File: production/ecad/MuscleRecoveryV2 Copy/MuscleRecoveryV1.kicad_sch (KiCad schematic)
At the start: 18 parts, among them J6 Screw_Terminal_01x06, U6 ESP32-WROOM-32E__16MB_

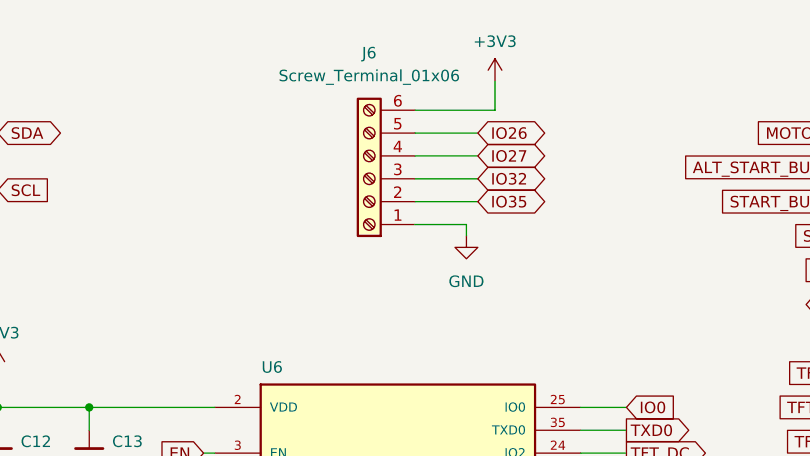
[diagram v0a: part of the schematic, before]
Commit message: Created New Layout
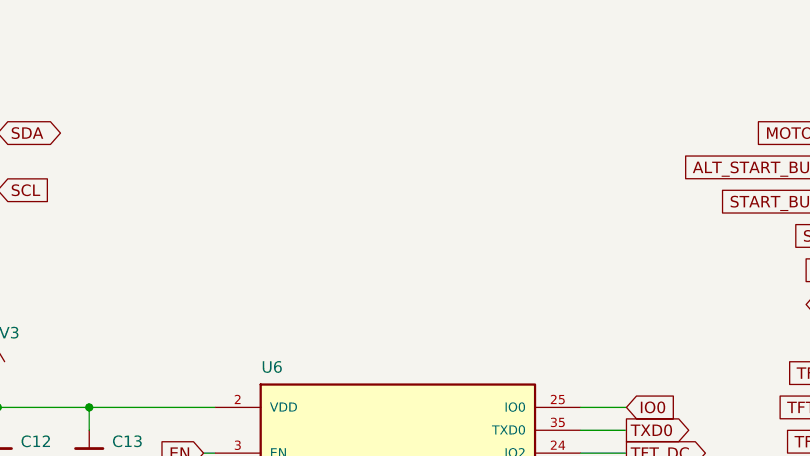
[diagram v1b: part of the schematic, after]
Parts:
- removed J6: Screw_Terminal_01x06, symbol Connector:Screw_Terminal_01x06
- C12, C13: footprint Capacitor_SMD:C_0805_2012Metric -> Capacitor_SMD:C_0402_1005Metric
- R30, R31, R34: footprint Resistor_SMD:R_0805_2012Metric -> Resistor_SMD:R_0402_1005Metric
- U6: footprint ESP32-WROOM-32E__16MB_:XCVR_ESP32-WROOM-32E__16MB_ -> Muscle_Recovery_Footprint_Library:XCVR_ESP32-WROOM-32E__16MB_
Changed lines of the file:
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@@
-    (stroke (width 0) (type default))
-  )
-  (wire (pts (xy 141.605 38.1) (xy 148.59 38.1))
     (stroke (width 0) (type default))
   )
@@
     (stroke (width 0) (type default))
   )
-  (wire (pts (xy 141.605 30.48) (xy 148.59 30.48))
-    (stroke (width 0) (type default))
-  )
-  (wire (pts (xy 150.495 27.94) (xy 150.495 24.765))
-    (stroke (width 0) (type default))
-  )
   (wire (pts (xy 160.02 101.6) (xy 165.1 101.6))
     (stroke (width 0) (type default))
   )
-  (wire (pts (xy 141.605 33.02) (xy 148.59 33.02))
-    (stroke (width 0) (type default))
-  )
   (wire (pts (xy 191.77 30.48) (xy 201.93 30.48))
     (stroke (width 0) (type default))
@@
     (stroke (width 0) (type default))
   )
-  (wire (pts (xy 147.32 40.64) (xy 147.32 41.91))
-    (stroke (width 0) (type default))
-  )
   (wire (pts (xy 185.42 85.09) (xy 186.69 85.09))
     (stroke (width 0) (type default))
@@
     (stroke (width 0) (type default))
   )
-  (wire (pts (xy 141.605 27.94) (xy 150.495 27.94))
-    (stroke (width 0) (type default))
-  )
   (wire (pts (xy 147.32 187.96) (xy 156.845 187.96))
     (stroke (width 0) (type default))
@@
     (stroke (width 0) (type default))
   )
-  (wire (pts (xy 141.605 40.64) (xy 147.32 40.64))
-    (stroke (width 0) (type default))
-  )
   (wire (pts (xy 186.69 96.52) (xy 193.04 96.52))
     (stroke (width 0) (type default))
@@
     (stroke (width 0) (type default))
   )
-  (wire (pts (xy 141.605 35.56) (xy 148.59 35.56))
-    (stroke (width 0) (type default))
-  )
   (wire (pts (xy 182.88 99.06) (xy 193.04 99.06))
     (stroke (width 0) (type default))
@@
     )
   )
-  (global_label "IO35" (shape bidirectional) (at 148.59 38.1 0) (fields_autoplaced)
-    (effects (font (size 1.27 1.27)) (justify left))
-    (property "Intersheetrefs" "${INTERSHEET_REFS}" (at 157.0408 38.1 0)
-      (effects (font (size 1.27 1.27)) (justify left) hide)
-    )
-  )
   (global_label "SD_CS" (shape output) (at 165.1 81.28 0) (fields_autoplaced)
     (effects (font (size 1.27 1.27)) (justify left))
@@
     )
   )
-  (global_label "IO32" (shape bidirectional) (at 148.59 35.56 0) (fields_autoplaced)
-    (effects (font (size 1.27 1.27)) (justify left))
-    (property "Intersheetrefs" "${INTERSHEET_REFS}" (at 157.0408 35.56 0)
-      (effects (font (size 1.27 1.27)) (justify left) hide)
-    )
-  )
   (global_label "RXD0" (shape output) (at 193.04 142.24 180) (fields_autoplaced)
     (effects (font (size 1.27 1.27)) (justify right))
@@
     )
   )
-  (global_label "IO27" (shape bidirectional) (at 148.59 33.02 0) (fields_autoplaced)
-    (effects (font (size 1.27 1.27)) (justify left))
-    (property "Intersheetrefs" "${INTERSHEET_REFS}" (at 157.0408 33.02 0)
-      (effects (font (size 1.27 1.27)) (justify left) hide)
-    )
-  )
   (global_label "SDA" (shape bidirectional) (at 95.25 30.48 0) (fields_autoplaced)
     (effects (font (size 1.27 1.27)) (justify left))
@@
     (effects (font (size 1.27 1.27)) (justify left))
     (property "Intersheetrefs" "${INTERSHEET_REFS}" (at 165.7568 187.96 0)
-      (effects (font (size 1.27 1.27)) (justify left) hide)
-    )
-  )
-  (global_label "IO26" (shape bidirectional) (at 148.59 30.48 0) (fields_autoplaced)
-    (effects (font (size 1.27 1.27)) (justify left))
-    (property "Intersheetrefs" "${INTERSHEET_REFS}" (at 157.0408 30.48 0)
       (effects (font (size 1.27 1.27)) (justify left) hide)
     )
@@
         (path "/4e550305-79d2-4e4a-a502-817ebcc79f9a"
           (reference "#PWR052") (unit 1)
-        )
-      )
-    )
-  )
-  (symbol (lib_id "power:GND") (at 147.32 41.91 0) (unit 1)
-    (in_bom yes) (on_board yes) (dnp no) (fields_autoplaced)
-    (property "Reference" "#PWR064" (at 147.32 48.26 0)
-      (effects (font (size 1.27 1.27)) hide)
-    )
-    (property "Value" "GND" (at 147.32 46.99 0)
-      (effects (font (size 1.27 1.27)))
-    )
-    (property "Footprint" "" (at 147.32 41.91 0)
-      (effects (font (size 1.27 1.27)) hide)
-    )
-    (property "Datasheet" "" (at 147.32 41.91 0)
-      (effects (font (size 1.27 1.27)) hide)
-    )
-    (pin "1")
-    (instances
-      (project "MuscleRecoveryV1"
-        (path "/4e550305-79d2-4e4a-a502-817ebcc79f9a"
-          (reference "#PWR064") (unit 1)
         )
       )
@@
       (effects (font (size 1.27 1.27)) (justify left))
     )
-    (property "Footprint" "Capacitor_SMD:C_0805_2012Metric" (at 95.25 66.04 0)
+    (property "Footprint" "Capacitor_SMD:C_0402_1005Metric" (at 95.25 66.04 0)
       (effects (font (size 1.27 1.27)) hide)
     )
@@
       (effects (font (size 1.27 1.27)) (justify left))
     )
-    (property "Footprint" "Capacitor_SMD:C_0805_2012Metric" (at 105.41 66.04 0)
+    (property "Footprint" "Capacitor_SMD:C_0402_1005Metric" (at 105.41 66.04 0)
       (effects (font (size 1.27 1.27)) hide)
     )
@@
     )
   )
-  (symbol (lib_id "power:+3V3") (at 150.495 24.765 0) (unit 1)
-    (in_bom yes) (on_board yes) (dnp no) (fields_autoplaced)
-    (property "Reference" "#PWR065" (at 150.495 28.575 0)
-      (effects (font (size 1.27 1.27)) hide)
-    )
-    (property "Value" "+3V3" (at 150.495 20.32 0)
-      (effects (font (size 1.27 1.27)))
-    )
-    (property "Footprint" "" (at 150.495 24.765 0)
-      (effects (font (size 1.27 1.27)) hide)
-    )
-    (property "Datasheet" "" (at 150.495 24.765 0)
-      (effects (font (size 1.27 1.27)) hide)
-    )
-    (pin "1")
-    (instances
-      (project "MuscleRecoveryV1"
-        (path "/4e550305-79d2-4e4a-a502-817ebcc79f9a"
-          (reference "#PWR065") (unit 1)
-        )
-      )
-    )
-  )
-  (symbol (lib_id "Connector:Screw_Terminal_01x06") (at 136.525 35.56 180) (unit 1)
-    (in_bom yes) (on_board yes) (dnp no) (fields_autoplaced)
-    (property "Reference" "J6" (at 136.525 21.59 0)
-      (effects (font (size 1.27 1.27)))
-    )
-    (property "Value" "Screw_Terminal_01x06" (at 136.525 24.13 0)
-      (effects (font (size 1.27 1.27)))
-    )
-    (property "Footprint" "" (at 136.525 35.56 0)
-      (effects (font (size 1.27 1.27)) hide)
-    )
-    (property "Datasheet" "~" (at 136.525 35.56 0)
-      (effects (font (size 1.27 1.27)) hide)
-    )
-    (pin "1")
-    (pin "2")
-    (pin "3")
-    (pin "4")
-    (pin "5")
-    (pin "6")
-    (instances
-      (project "MuscleRecoveryV1"
-        (path "/4e550305-79d2-4e4a-a502-817ebcc79f9a"
-          (reference "J6") (unit 1)
-        )
-      )
-    )
-  )
   (symbol (lib_id "Device:R") (at 186.69 91.44 0) (unit 1)
     (in_bom yes) (on_board yes) (dnp no) (fields_autoplaced)
@@
       (effects (font (size 1.27 1.27)) (justify left))
     )
-    (property "Footprint" "Resistor_SMD:R_0805_2012Metric" (at 184.912 91.44 90)
+    (property "Footprint" "Resistor_SMD:R_0402_1005Metric" (at 184.912 91.44 90)
       (effects (font (size 1.27 1.27)) hide)
     )
@@
       (effects (font (size 1.27 1.27)) (justify right))
     )
-    (property "Footprint" "Resistor_SMD:R_0805_2012Metric" (at 184.658 91.44 90)
+    (property "Footprint" "Resistor_SMD:R_0402_1005Metric" (at 184.658 91.44 90)
       (effects (font (size 1.27 1.27)) hide)
     )
@@
       (effects (font (size 1.27 1.27)))
     )
-    (property "Footprint" "Resistor_SMD:R_0805_2012Metric" (at 165.1 69.342 90)
+    (property "Footprint" "Resistor_SMD:R_0402_1005Metric" (at 165.1 69.342 90)
       (effects (font (size 1.27 1.27)) hide)
     )
@@
       (effects (font (size 1.27 1.27)))
     )
-    (property "Footprint" "ESP32-WROOM-32E__16MB_:XCVR_ESP32-WROOM-32E__16MB_" (at 143.51 144.78 0)
+    (property "Footprint" "Muscle_Recovery_Footprint_Library:XCVR_ESP32-WROOM-32E__16MB_" (at 143.51 144.78 0)
       (effects (font (size 1.27 1.27)) (justify bottom) hide)
     )

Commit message: Committing My pliminary placement for my PCB <3
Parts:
- C12, C13: footprint Capacitor_SMD:C_0402_1005Metric -> Capacitor_SMD:C_0805_2012Metric
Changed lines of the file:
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@@
       (effects (font (size 1.27 1.27)) (justify left))
     )
-    (property "Footprint" "Capacitor_SMD:C_0402_1005Metric" (at 95.25 66.04 0)
+    (property "Footprint" "Capacitor_SMD:C_0805_2012Metric" (at 95.25 66.04 0)
       (effects (font (size 1.27 1.27)) hide)
     )
@@
       (effects (font (size 1.27 1.27)) (justify left))
     )
-    (property "Footprint" "Capacitor_SMD:C_0402_1005Metric" (at 105.41 66.04 0)
+    (property "Footprint" "Capacitor_SMD:C_0805_2012Metric" (at 105.41 66.04 0)
       (effects (font (size 1.27 1.27)) hide)
     )

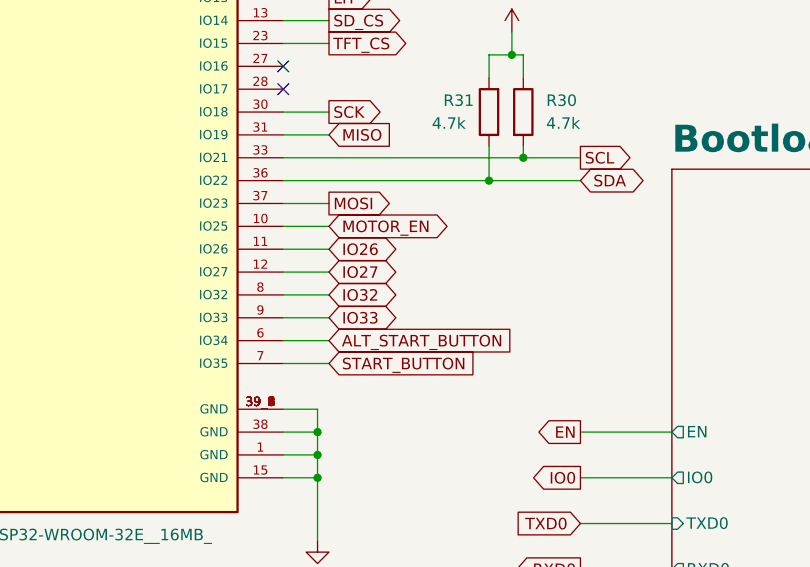
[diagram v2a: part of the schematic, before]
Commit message: committing some recent changes to layout
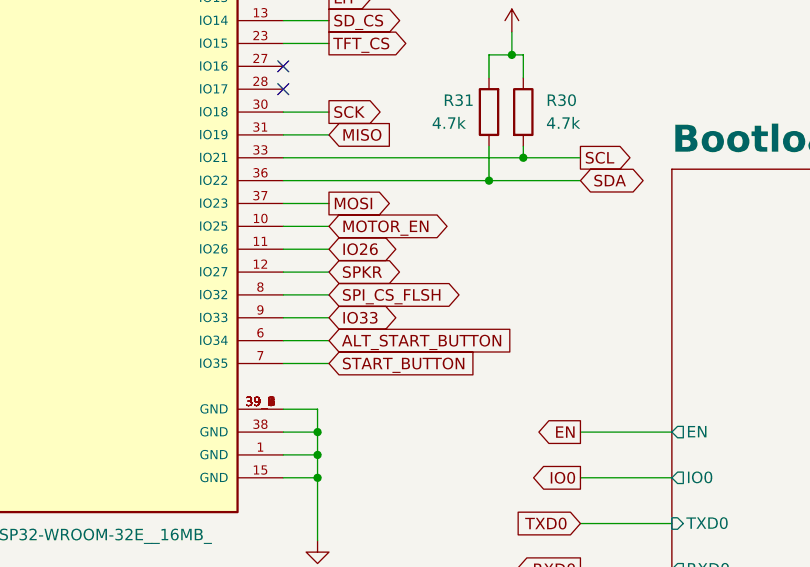
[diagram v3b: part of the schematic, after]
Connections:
- net IO27 renamed SPKR
- net IO32 renamed SPI_CS_FLSH
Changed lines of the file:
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@@
     )
   )
-  (global_label "IO32" (shape bidirectional) (at 165.1 111.76 0) (fields_autoplaced)
+  (global_label "SPI_CS_FLSH" (shape bidirectional) (at 165.1 111.76 0) (fields_autoplaced)
     (effects (font (size 1.27 1.27)) (justify left))
-    (property "Intersheetrefs" "${INTERSHEET_REFS}" (at 173.5508 111.76 0)
+    (property "Intersheetrefs" "${INTERSHEET_REFS}" (at 181.3522 111.76 0)
       (effects (font (size 1.27 1.27)) (justify left) hide)
     )
@@
     )
   )
-  (global_label "IO27" (shape bidirectional) (at 165.1 109.22 0) (fields_autoplaced)
+  (global_label "SPKR" (shape bidirectional) (at 165.1 109.22 0) (fields_autoplaced)
     (effects (font (size 1.27 1.27)) (justify left))
-    (property "Intersheetrefs" "${INTERSHEET_REFS}" (at 173.5508 109.22 0)
+    (property "Intersheetrefs" "${INTERSHEET_REFS}" (at 174.216 109.22 0)
       (effects (font (size 1.27 1.27)) (justify left) hide)
     )

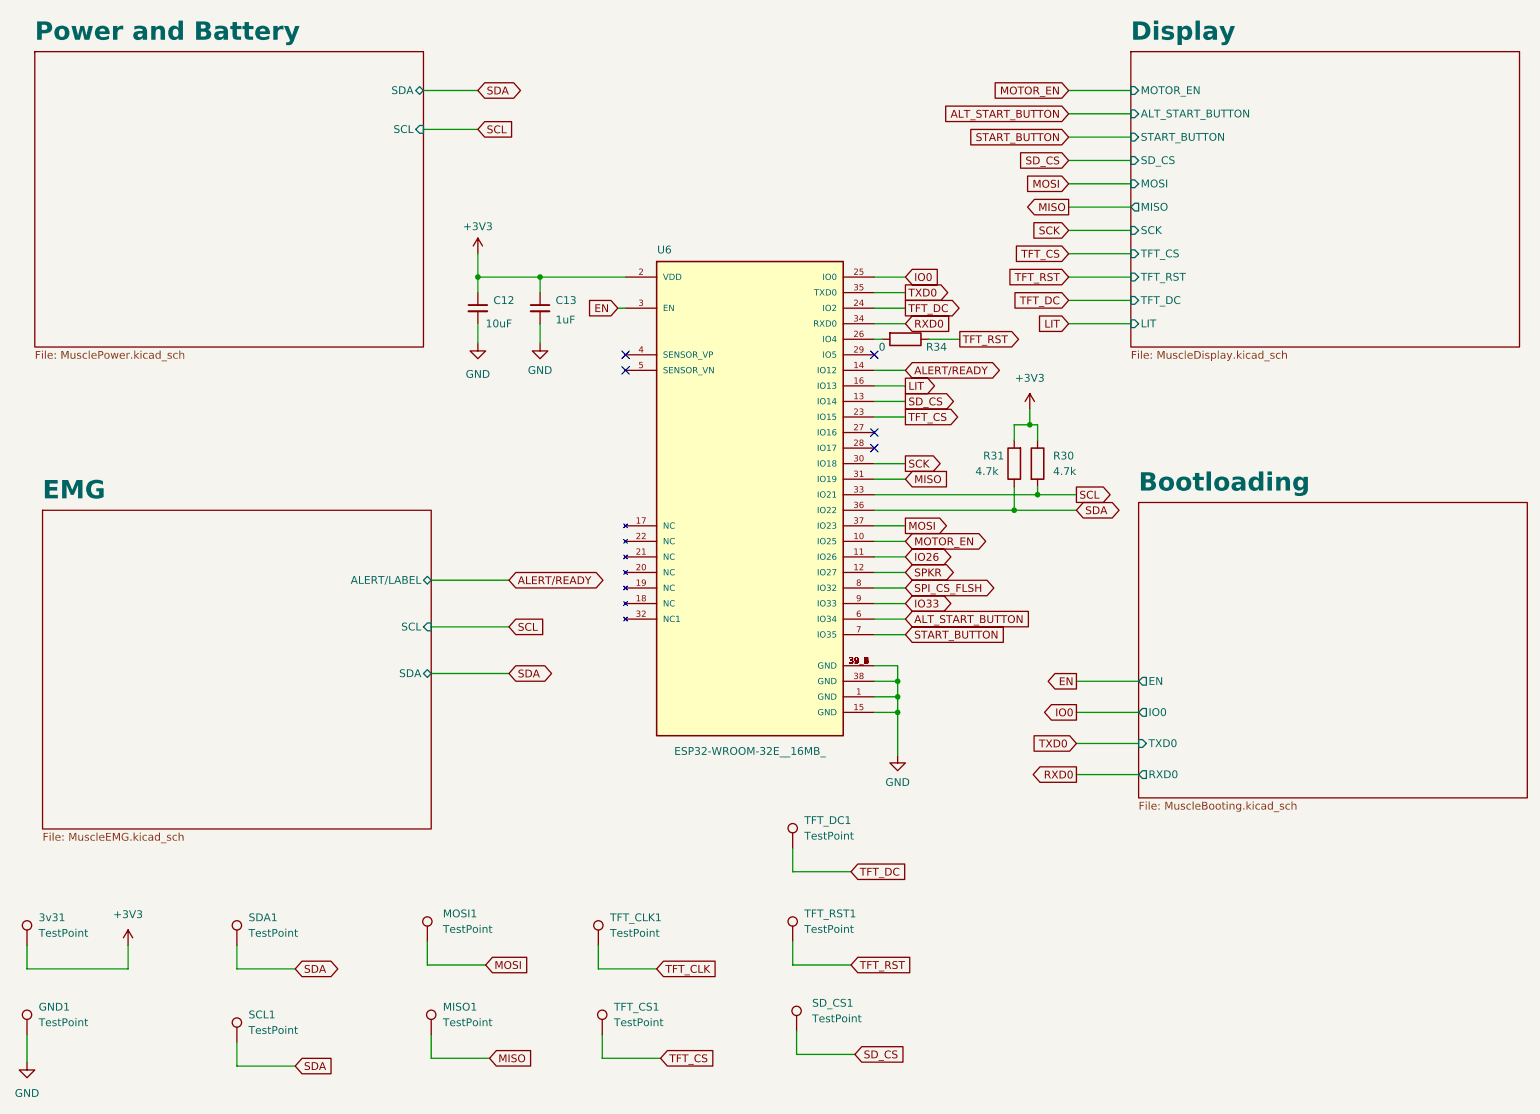
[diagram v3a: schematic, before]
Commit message: Pushing Most of the final changes for PCB REV2
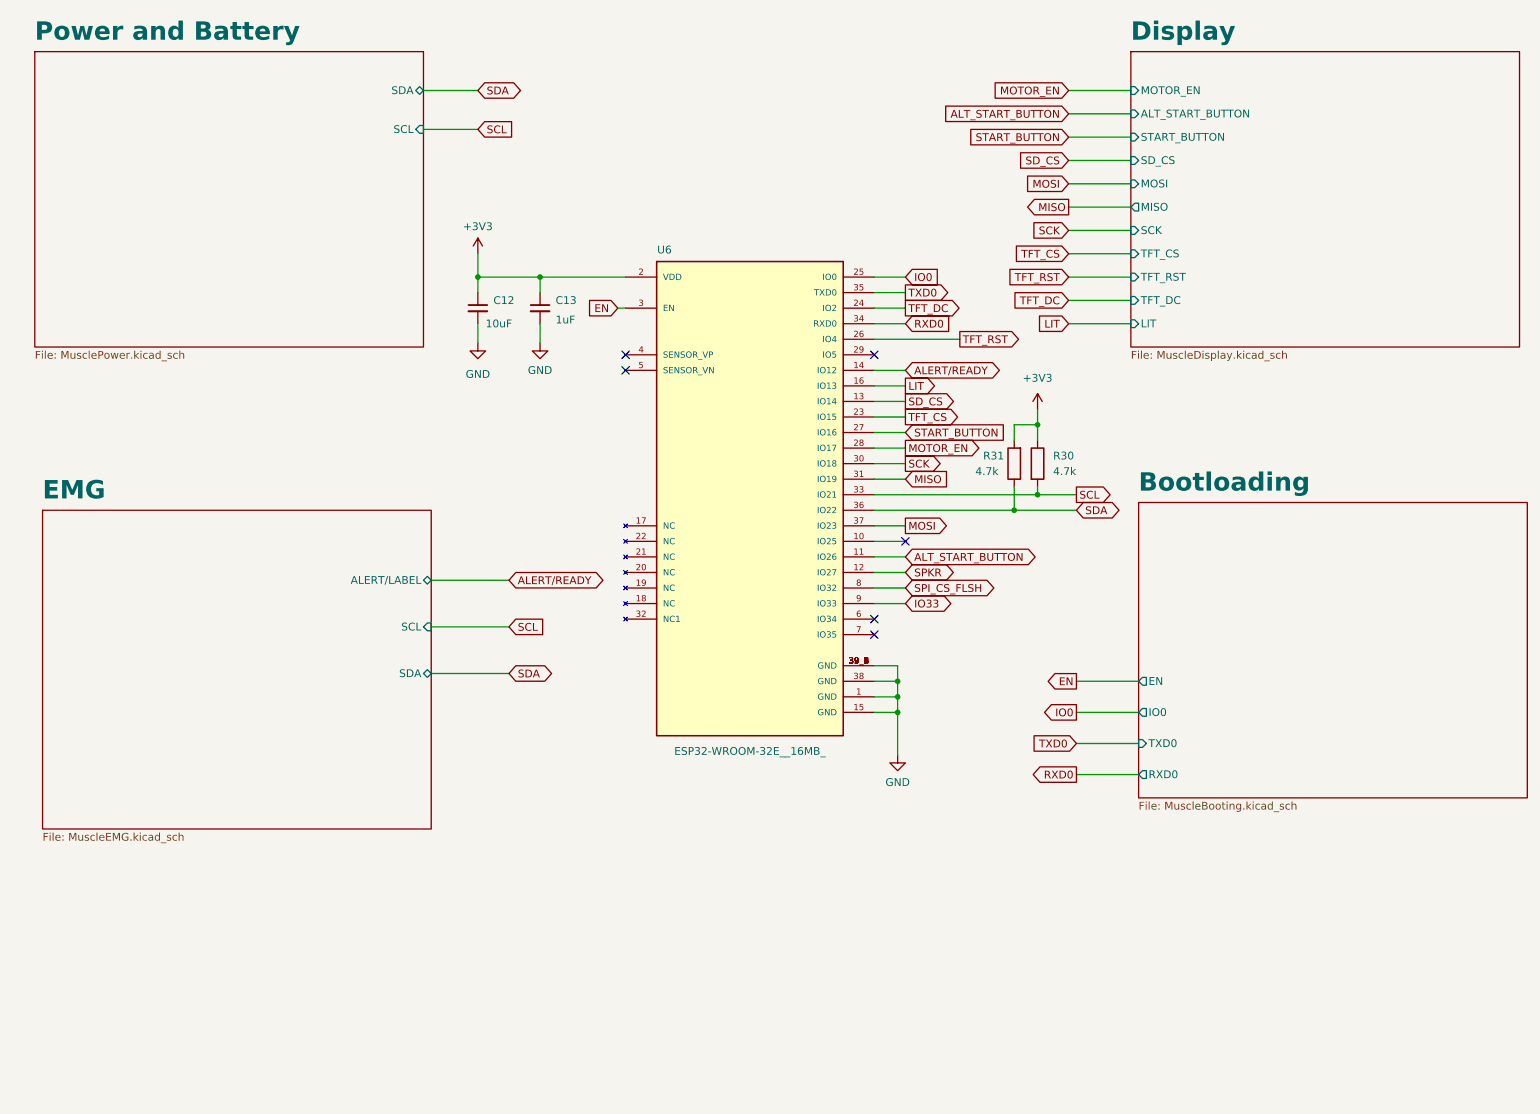
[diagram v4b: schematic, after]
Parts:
- removed 3v31, GND1, MISO1, MOSI1, SCL1, SDA1, SD_CS1, TFT_CLK1, TFT_CS1, TFT_DC1, TFT_RST1: TestPoint, TestPoint:TestPoint_Pad_D1.5mm, symbol Connector:TestPoint
- removed R34: 0, Resistor_SMD:R_0402_1005Metric, symbol Device:R
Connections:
- net IO26 is gone; now on net ALT_START_BUTTON: U6.11 (IO26)
- net ALT_START_BUTTON: no longer U6.6 (IO34)
- net MOTOR_EN: now also U6.28 (IO17); no longer U6.10 (IO25)
- net START_BUTTON: now also U6.27 (IO16); no longer U6.7 (IO35)
- net TFT_RST: now also U6.26 (IO4)
- no-connect marks 5 -> 6
